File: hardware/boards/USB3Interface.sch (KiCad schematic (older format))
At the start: 3 parts, among them J2 USB3_Micro_B_Amphenol, U1 ECP5UM5G-381caBGA, U3 CYUSB3014

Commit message: Some more mist schematic edits
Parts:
- J2: DIGIKEY_PN (none) -> GSB343K33HRCT-ND
- U1: DIGIKEY_PN (none) -> 220-2112-ND
- U3: DIGIKEY_PN (none) -> 428-3130-ND
- U3: DIGIKEY_PN (none) -> 428-3130-ND; MPN https://www.cypress.com/file/140296/download -> CYUSB3014-BZXI
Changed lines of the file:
@@
 F 4 "Lattice" H 9800 1200 50  0001 C CNN "MFR"
 F 5 "LFE5UM5G-85F-8BG381I" H 9800 1200 50  0001 C CNN "MPN"
+F 6 "220-2112-ND" H 9800 1200 50  0001 C CNN "DIGIKEY_PN"
 	3    9800 1200
 	1    0    0    -1
@@
 F 4 "Cypress" H 6400 3350 50  0001 C CNN "MFR"
 F 5 " CYUSB3014-BZXI" H 6400 3350 50  0001 C CNN "MPN"
+F 6 "428-3130-ND" H 6400 3350 50  0001 C CNN "DIGIKEY_PN"
 	2    6400 3350
 	1    0    0    -1
@@
 F 4 "Cypress" H 3050 1700 50  0001 C CNN "MFR"
 F 5 " CYUSB3014-BZXI" H 3050 1700 50  0001 C CNN "MPN"
+F 6 "428-3130-ND" H 3050 1700 50  0001 C CNN "DIGIKEY_PN"
 	3    3050 1700
 	1    0    0    -1
@@
 F 3 "https://www.cypress.com/file/140296/download" H 6950 2100 50  0001 C CNN
 F 4 "Cypress" H 6950 1400 50  0001 C CNN "MFR"
-F 5 "https://www.cypress.com/file/140296/download" H 6950 1400 50  0001 C CNN "MPN"
+F 5 " CYUSB3014-BZXI" H 6950 1400 50  0001 C CNN "MPN"
+F 6 "428-3130-ND" H 6950 1400 50  0001 C CNN "DIGIKEY_PN"
 	4    6950 1400
 	1    0    0    -1
@@
 F 4 "Amphenol" H 3050 3050 50  0001 C CNN "MFR"
 F 5 "GSB343K33HR" H 3050 3050 50  0001 C CNN "MPN"
+F 6 "GSB343K33HRCT-ND" H 3050 2600 50  0001 C CNN "DIGIKEY_PN"
 	1    3050 2600
 	1    0    0    -1

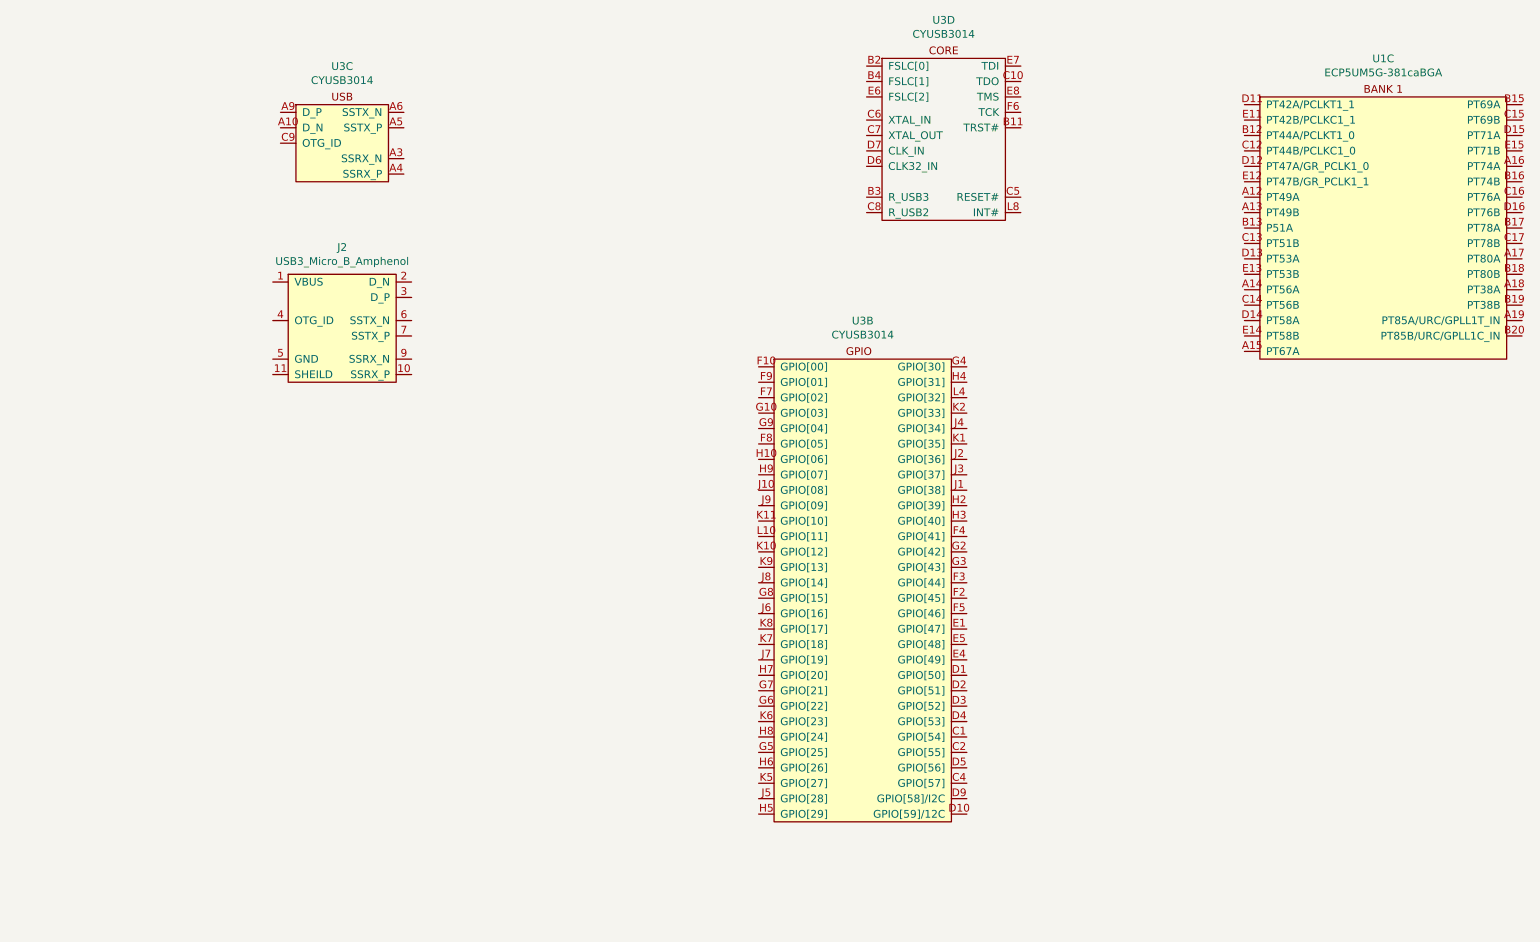
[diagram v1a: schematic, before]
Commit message: Lots of small updates, getting values specified for parts, switched the BJT to NFETs
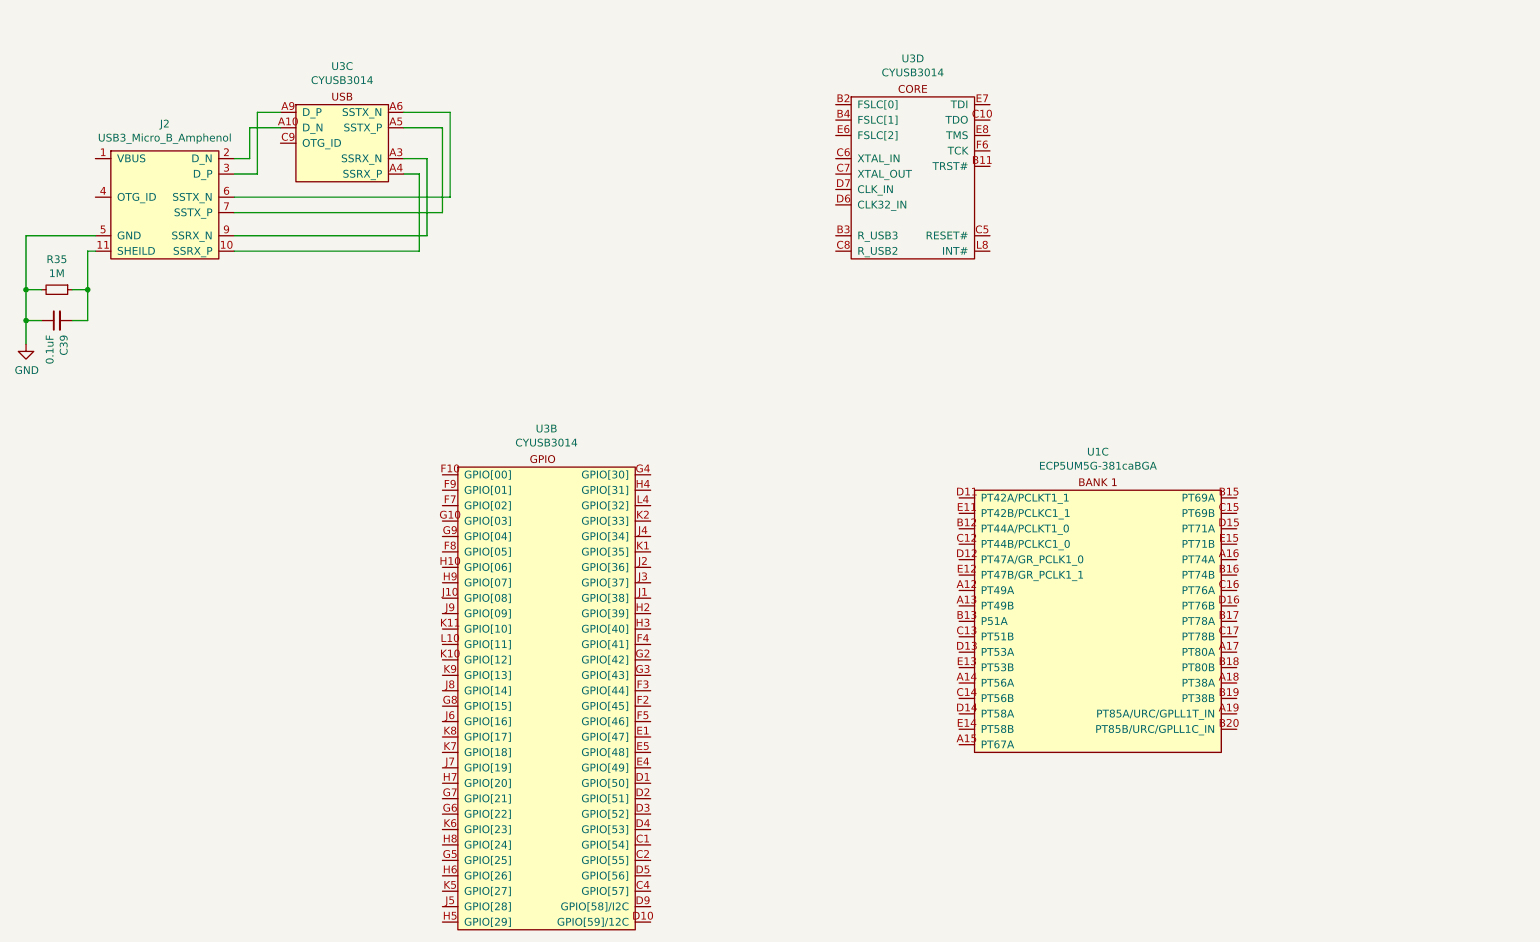
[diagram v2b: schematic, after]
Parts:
- added C39: 0.1uF, Capacitor_SMD:C_0603_1608Metric, symbol Device:C_Small
- added R35: 1M, Resistor_SMD:R_0603_1608Metric, symbol Device:R_Small
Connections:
- net at U3.A10 (D_N): now also J2.2 (D_N)
- net at U3.A3 (SSRX_N): now also J2.9 (SSRX_N)
- net at U3.A4 (SSRX_P): now also J2.10 (SSRX_P)
- net at U3.A5 (SSTX_P): now also J2.7 (SSTX_P)
- net at U3.A6 (SSTX_N): now also J2.6 (SSTX_N)
- net at U3.A9 (D_P): now also J2.3 (D_P)
- net at J2.11 (SHEILD): now also C39.2, R35.1
- net GND: now reaches J2.5 (GND), J2.8 (GND)
- net GND: now also C39.1, R35.2
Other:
- moved on the sheet: J2, U1C, U3B, U3D
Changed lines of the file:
@@
 $Descr A4 11693 8268
 encoding utf-8
-Sheet 10 11
+Sheet 7 10
 Title ""
 Date ""
@@
 L lethalbit:ECP5UM5G-381caBGA U?
 U 3 1 5F2EB784
-P 9800 1200
+P 7950 3750
 AR Path="/5F2EB784" Ref="U?"  Part="3"
 AR Path="/5F2CAFD2/5F2EB784" Ref="U1"  Part="3"
-F 0 "U1" H 9800 1548 50  0000 C CNN
-F 1 "ECP5UM5G-381caBGA" H 9800 1457 50  0000 C CNN
-F 2 "lethalbit:318caBGA" H 8450 1350 50  0001 C CNN
-F 3 "" H 8450 1350 50  0001 C CNN
-F 4 "Lattice" H 9800 1200 50  0001 C CNN "MFR"
-F 5 "LFE5UM5G-85F-8BG381I" H 9800 1200 50  0001 C CNN "MPN"
-F 6 "220-2112-ND" H 9800 1200 50  0001 C CNN "DIGIKEY_PN"
-	3    9800 1200
+F 0 "U1" H 7950 4098 50  0000 C CNN
+F 1 "ECP5UM5G-381caBGA" H 7950 4007 50  0000 C CNN
+F 2 "lethalbit:318caBGA" H 6600 3900 50  0001 C CNN
+F 3 "" H 6600 3900 50  0001 C CNN
+F 4 "Lattice" H 7950 3750 50  0001 C CNN "MFR"
+F 5 "LFE5UM5G-85F-8BG381I" H 7950 3750 50  0001 C CNN "MPN"
+F 6 "220-2112-ND" H 7950 3750 50  0001 C CNN "DIGIKEY_PN"
+	3    7950 3750
 	1    0    0    -1
 $EndComp
@@
 L lethalbit:CYUSB3014 U3
 U 2 1 5F3318A9
-P 6400 3350
-F 0 "U3" H 6425 4148 50  0000 C CNN
-F 1 "CYUSB3014" H 6425 4057 50  0000 C CNN
-F 2 "lethalbit:BGA-121_11x11_10.0x10.0mm" H 6400 4050 50  0001 C CNN
-F 3 "https://www.cypress.com/file/140296/download" H 6400 4050 50  0001 C CNN
-F 4 "Cypress" H 6400 3350 50  0001 C CNN "MFR"
-F 5 " CYUSB3014-BZXI" H 6400 3350 50  0001 C CNN "MPN"
-F 6 "428-3130-ND" H 6400 3350 50  0001 C CNN "DIGIKEY_PN"
-	2    6400 3350
+P 4350 4050
+F 0 "U3" H 4375 4848 50  0000 C CNN
+F 1 "CYUSB3014" H 4375 4757 50  0000 C CNN
+F 2 "lethalbit:BGA-121_11x11_10.0x10.0mm" H 4350 4750 50  0001 C CNN
+F 3 "https://www.cypress.com/file/140296/download" H 4350 4750 50  0001 C CNN
+F 4 "Cypress" H 4350 4050 50  0001 C CNN "MFR"
+F 5 " CYUSB3014-BZXI" H 4350 4050 50  0001 C CNN "MPN"
+F 6 "428-3130-ND" H 4350 4050 50  0001 C CNN "DIGIKEY_PN"
+	2    4350 4050
 	1    0    0    -1
 $EndComp
@@
 L lethalbit:CYUSB3014 U3
 U 4 1 5F335021
-P 6950 1400
-F 0 "U3" H 6950 2198 50  0000 C CNN
-F 1 "CYUSB3014" H 6950 2107 50  0000 C CNN
-F 2 "lethalbit:BGA-121_11x11_10.0x10.0mm" H 6950 2100 50  0001 C CNN
-F 3 "https://www.cypress.com/file/140296/download" H 6950 2100 50  0001 C CNN
-F 4 "Cypress" H 6950 1400 50  0001 C CNN "MFR"
-F 5 " CYUSB3014-BZXI" H 6950 1400 50  0001 C CNN "MPN"
-F 6 "428-3130-ND" H 6950 1400 50  0001 C CNN "DIGIKEY_PN"
-	4    6950 1400
+P 6750 1650
+F 0 "U3" H 6750 2448 50  0000 C CNN
+F 1 "CYUSB3014" H 6750 2357 50  0000 C CNN
+F 2 "lethalbit:BGA-121_11x11_10.0x10.0mm" H 6750 2350 50  0001 C CNN
+F 3 "https://www.cypress.com/file/140296/download" H 6750 2350 50  0001 C CNN
+F 4 "Cypress" H 6750 1650 50  0001 C CNN "MFR"
+F 5 " CYUSB3014-BZXI" H 6750 1650 50  0001 C CNN "MPN"
+F 6 "428-3130-ND" H 6750 1650 50  0001 C CNN "DIGIKEY_PN"
+	4    6750 1650
 	1    0    0    -1
 $EndComp
@@
 L lethalbit:USB3_Micro_B_Amphenol J2
 U 1 1 5F8A43B9
-P 3050 2600
-F 0 "J2" H 3050 3125 50  0000 C CNN
-F 1 "USB3_Micro_B_Amphenol" H 3050 3034 50  0000 C CNN
-F 2 "lethalbit:USB3_Micro_B_Amphenol" H 3050 3050 50  0001 C CNN
-F 3 "https://www.amphenol-icc.com/media/wysiwyg/files/drawing/gsb343k33hr.pdf" H 3050 3050 50  0001 C CNN
-F 4 "Amphenol" H 3050 3050 50  0001 C CNN "MFR"
-F 5 "GSB343K33HR" H 3050 3050 50  0001 C CNN "MPN"
-F 6 "GSB343K33HRCT-ND" H 3050 2600 50  0001 C CNN "DIGIKEY_PN"
-	1    3050 2600
+P 1900 1800
+F 0 "J2" H 1900 2325 50  0000 C CNN
+F 1 "USB3_Micro_B_Amphenol" H 1900 2234 50  0000 C CNN
+F 2 "lethalbit:USB3_Micro_B_Amphenol" H 1900 2250 50  0001 C CNN
+F 3 "https://www.amphenol-icc.com/media/wysiwyg/files/drawing/gsb343k33hr.pdf" H 1900 2250 50  0001 C CNN
+F 4 "Amphenol" H 1900 2250 50  0001 C CNN "MFR"
+F 5 "GSB343K33HR" H 1900 2250 50  0001 C CNN "MPN"
+F 6 "GSB343K33HRCT-ND" H 1900 1800 50  0001 C CNN "DIGIKEY_PN"
+	1    1900 1800
 	1    0    0    -1
 $EndComp
+Wire Wire Line
+	3450 1200 3750 1200
+Wire Wire Line
+	3750 1200 3750 1750
+Wire Wire Line
+	3750 1750 2350 1750
+Wire Wire Line
+	2350 1850 3700 1850
+Wire Wire Line
+	3700 1850 3700 1300
+Wire Wire Line
+	3700 1300 3450 1300
+Wire Wire Line
+	3450 1500 3600 1500
+Wire Wire Line
+	3600 1500 3600 2000
+Wire Wire Line
+	3600 2000 2350 2000
+Wire Wire Line
+	2350 1500 2450 1500
+Wire Wire Line
+	2450 1500 2450 1300
+Wire Wire Line
+	2450 1300 2650 1300
+Wire Wire Line
+	2350 1600 2500 1600
+Wire Wire Line
+	2500 1600 2500 1200
+Wire Wire Line
+	2500 1200 2650 1200
+Wire Wire Line
+	3450 1600 3550 1600
+Wire Wire Line
+	3550 1600 3550 2100
+Wire Wire Line
+	2350 2100 3550 2100
+$Comp
+L power:GND #PWR0118
+U 1 1 5EDDAAAC
+P 1000 2700
+F 0 "#PWR0118" H 1000 2450 50  0001 C CNN
+F 1 "GND" H 1005 2527 50  0000 C CNN
+F 2 "" H 1000 2700 50  0001 C CNN
+F 3 "" H 1000 2700 50  0001 C CNN
+	1    1000 2700
+	1    0    0    -1
+$EndComp
+Wire Wire Line
+	1450 2000 1000 2000
+Wire Wire Line
+	1000 2000 1000 2350
+$Comp
+L Device:R_Small R?
+U 1 1 5EDFF9C0
+P 1200 2350
+AR Path="/5EDF9F51/5EDFF9C0" Ref="R?"  Part="1"
+AR Path="/5F2CAFD2/5EDFF9C0" Ref="R35"  Part="1"
+F 0 "R35" V 1004 2350 50  0000 C CNN
+F 1 "1M" V 1095 2350 50  0000 C CNN
+F 2 "Resistor_SMD:R_0603_1608Metric" H 1200 2350 50  0001 C CNN
+F 3 "~" H 1200 2350 50  0001 C CNN
+F 4 "Vishay Dale" V 1200 2350 50  0001 C CNN "MFR"
+F 5 "CRCW06031M00FKEA" V 1200 2350 50  0001 C CNN "MPN"
+	1    1200 2350
+	0    1    1    0
+$EndComp
+$Comp
+L Device:C_Small C?
+U 1 1 5EDFF9C8
+P 1200 2550
+AR Path="/5EDF9F51/5EDFF9C8" Ref="C?"  Part="1"
+AR Path="/5F2CAFD2/5EDFF9C8" Ref="C39"  Part="1"
+F 0 "C39" H 1108 2504 50  0000 R CNN
+F 1 "0.1uF" H 1108 2595 50  0000 R CNN
+F 2 "Capacitor_SMD:C_0603_1608Metric" H 1200 2550 50  0001 C CNN
+F 3 "~" H 1200 2550 50  0001 C CNN
+F 4 "KEMET" V 1200 2550 50  0001 C CNN "MFR"
+F 5 "C0603C104M5RACTU" V 1200 2550 50  0001 C CNN "MPN"
+	1    1200 2550
+	0    -1   -1   0
+$EndComp
+Wire Wire Line
+	1100 2550 1000 2550
+Connection ~ 1000 2550
+Wire Wire Line
+	1000 2550 1000 2700
+Wire Wire Line
+	1100 2350 1000 2350
+Connection ~ 1000 2350
+Wire Wire Line
+	1000 2350 1000 2550
+Wire Wire Line
+	1450 2100 1400 2100
+Wire Wire Line
+	1400 2100 1400 2350
+Wire Wire Line
+	1400 2550 1300 2550
+Wire Wire Line
+	1300 2350 1400 2350
+Connection ~ 1400 2350
+Wire Wire Line
+	1400 2350 1400 2550
 $EndSCHEMATC
